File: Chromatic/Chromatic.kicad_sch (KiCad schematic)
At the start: 154 parts

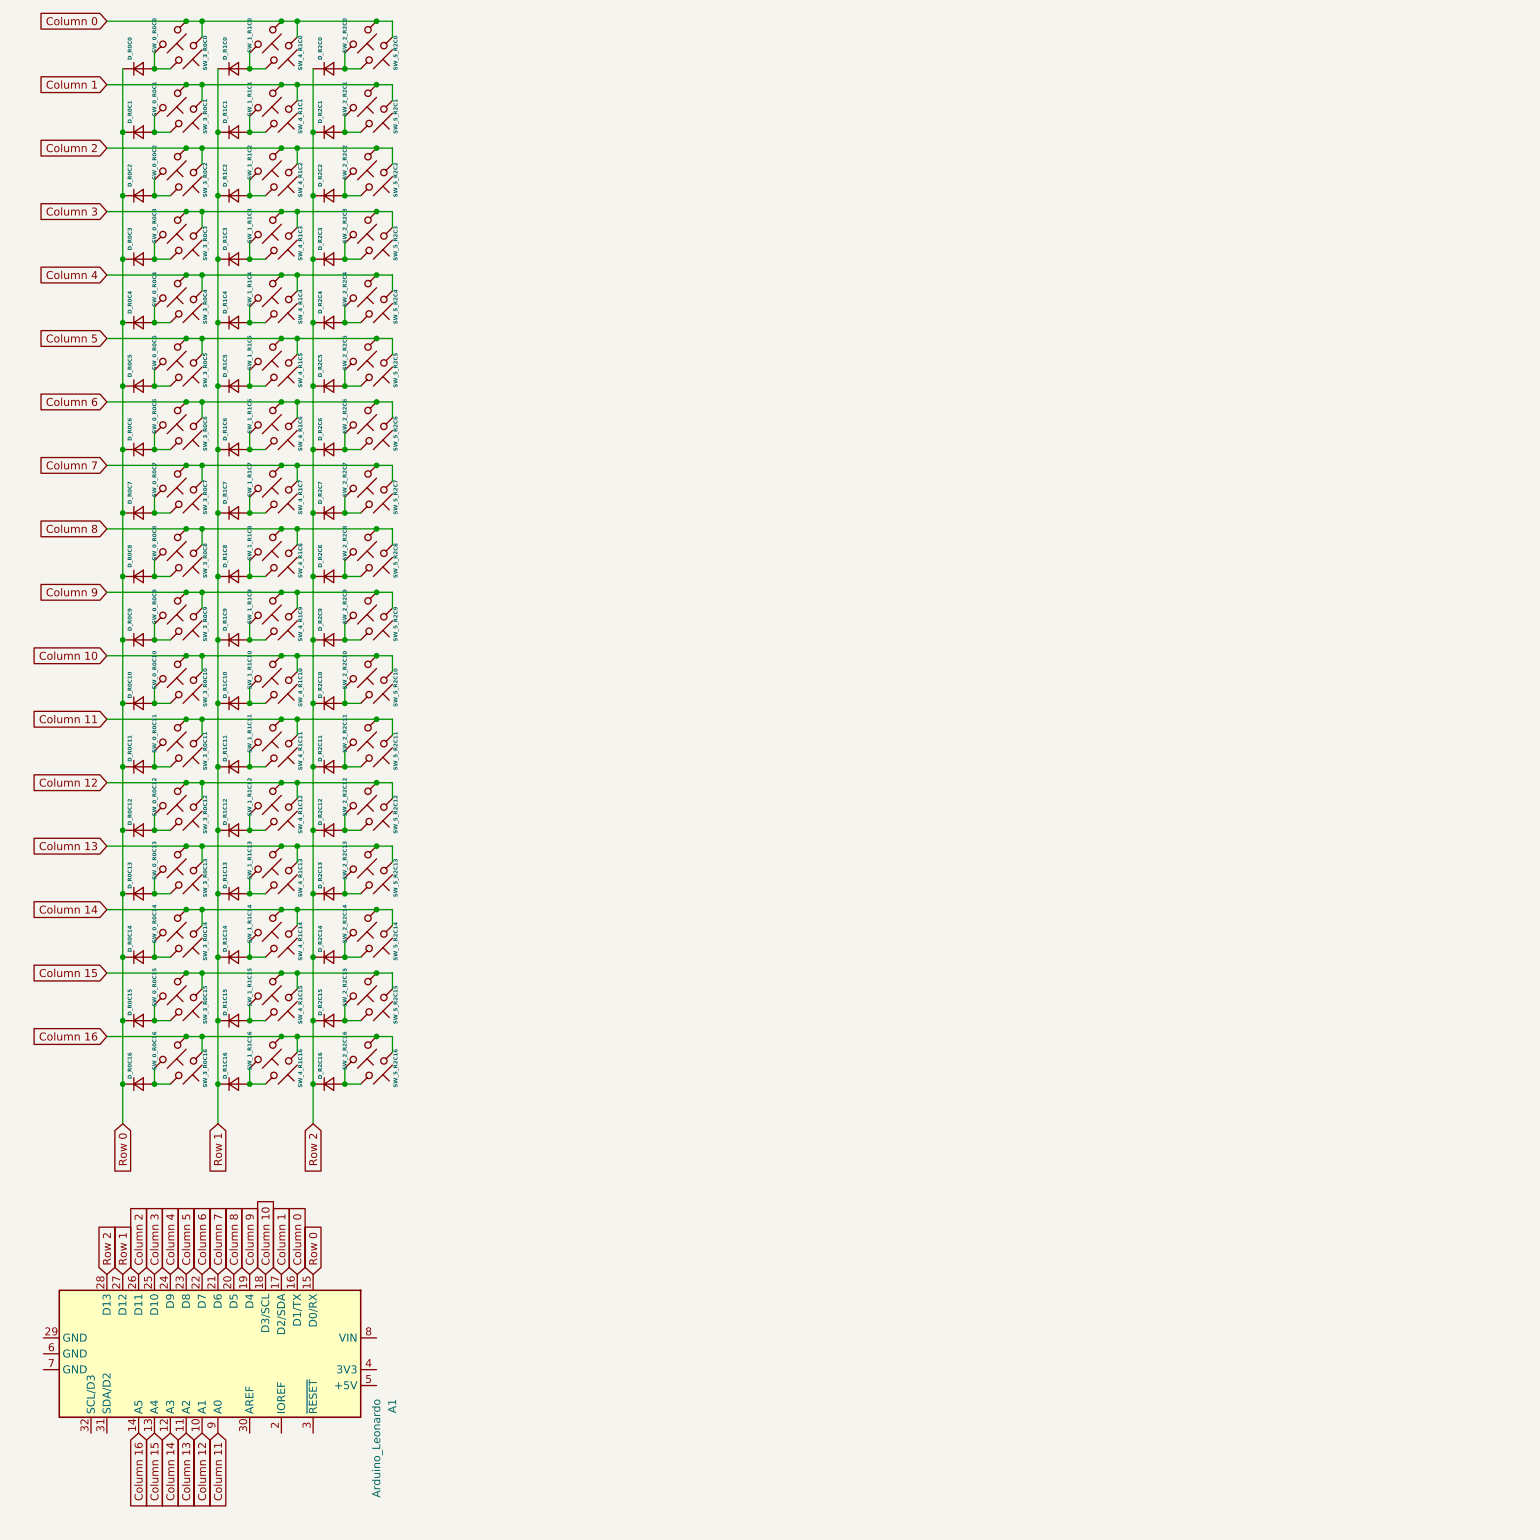
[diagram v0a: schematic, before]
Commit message: octave adjust
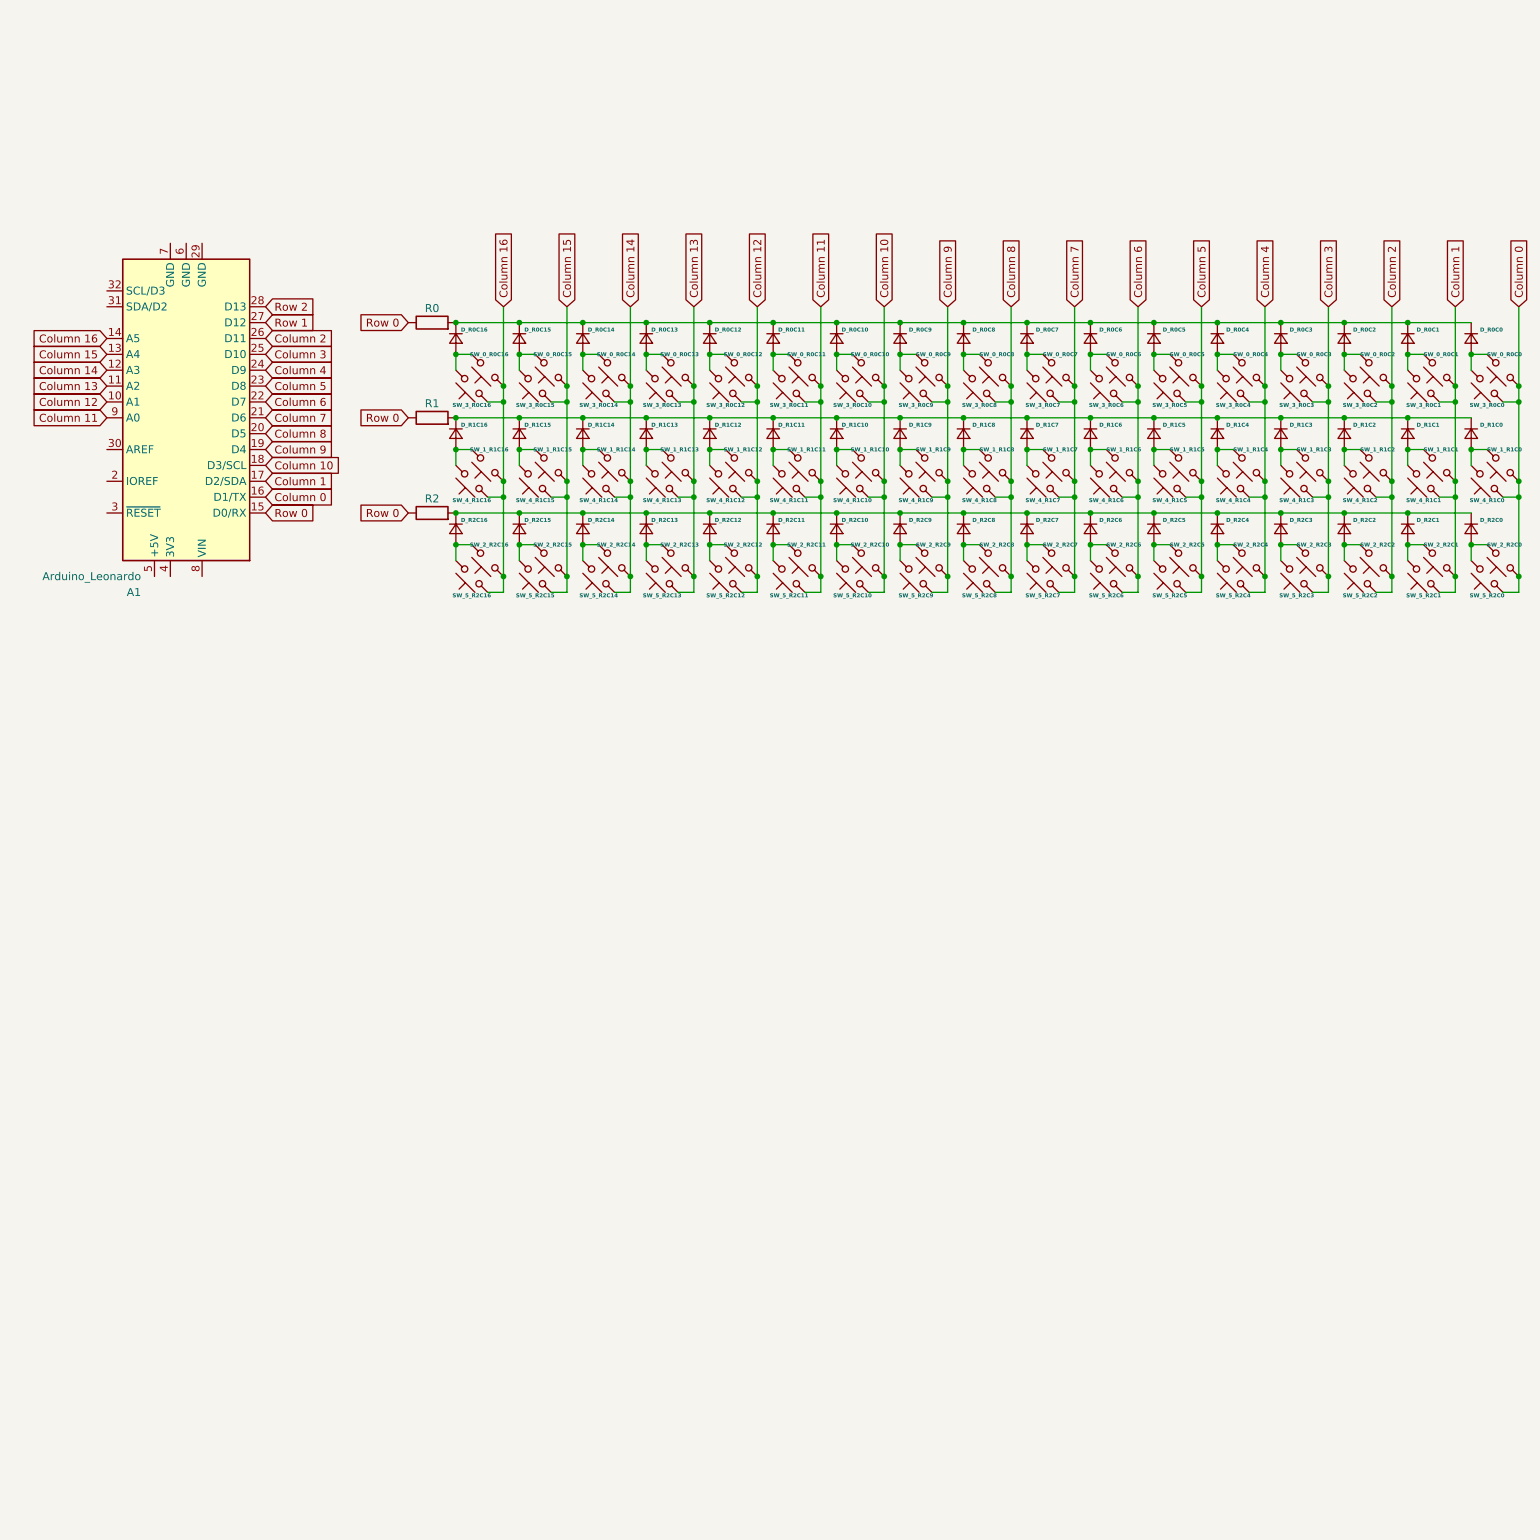
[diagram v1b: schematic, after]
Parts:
- added R0, R1, R2: Resistor, Resistor_THT:R_Axial_DIN0204_L3.6mm_D1.6mm_P5.08mm_Horizontal, symbol ScottoKeebs:Placeholder_Resistor
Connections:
- net Row 0: now also R0.1, R1.1, R2.1; no longer D_R0C0.1 (K), D_R0C1.1 (K), D_R0C10.1 (K), D_R0C11.1 (K), D_R0C12.1 (K), D_R0C13.1 (K), D_R0C14.1 (K), D_R0C15.1 (K), D_R0C16.1 (K), D_R0C2.1 (K), D_R0C3.1 (K), D_R0C4.1 (K), D_R0C5.1 (K), D_R0C6.1 (K), D_R0C7.1 (K), D_R0C8.1 (K), D_R0C9.1 (K)
- net Row 1: no longer D_R1C0.1 (K), D_R1C1.1 (K), D_R1C10.1 (K), D_R1C11.1 (K), D_R1C12.1 (K), D_R1C13.1 (K), D_R1C14.1 (K), D_R1C15.1 (K), D_R1C16.1 (K), D_R1C2.1 (K), D_R1C3.1 (K), D_R1C4.1 (K), D_R1C5.1 (K), D_R1C6.1 (K), D_R1C7.1 (K), D_R1C8.1 (K), D_R1C9.1 (K)
- net Row 2: no longer D_R2C0.1 (K), D_R2C1.1 (K), D_R2C10.1 (K), D_R2C11.1 (K), D_R2C12.1 (K), D_R2C13.1 (K), D_R2C14.1 (K), D_R2C15.1 (K), D_R2C16.1 (K), D_R2C2.1 (K), D_R2C3.1 (K), D_R2C4.1 (K), D_R2C5.1 (K), D_R2C6.1 (K), D_R2C7.1 (K), D_R2C8.1 (K), D_R2C9.1 (K)
- new net: D_R2C0.1 (K), D_R2C1.1 (K), D_R2C10.1 (K), D_R2C11.1 (K), D_R2C12.1 (K), D_R2C13.1 (K), D_R2C14.1 (K), D_R2C15.1 (K), D_R2C16.1 (K), D_R2C2.1 (K), D_R2C3.1 (K), D_R2C4.1 (K), D_R2C5.1 (K), D_R2C6.1 (K), D_R2C7.1 (K), D_R2C8.1 (K), D_R2C9.1 (K), R2.2
- new net: D_R0C0.1 (K), D_R0C1.1 (K), D_R0C10.1 (K), D_R0C11.1 (K), D_R0C12.1 (K), D_R0C13.1 (K), D_R0C14.1 (K), D_R0C15.1 (K), D_R0C16.1 (K), D_R0C2.1 (K), D_R0C3.1 (K), D_R0C4.1 (K), D_R0C5.1 (K), D_R0C6.1 (K), D_R0C7.1 (K), D_R0C8.1 (K), D_R0C9.1 (K), R0.2
- new net: D_R1C0.1 (K), D_R1C1.1 (K), D_R1C10.1 (K), D_R1C11.1 (K), D_R1C12.1 (K), D_R1C13.1 (K), D_R1C14.1 (K), D_R1C15.1 (K), D_R1C16.1 (K), D_R1C2.1 (K), D_R1C3.1 (K), D_R1C4.1 (K), D_R1C5.1 (K), D_R1C6.1 (K), D_R1C7.1 (K), D_R1C8.1 (K), D_R1C9.1 (K), R1.2
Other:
- moved on the sheet: A1, D_R0C0, D_R0C1, D_R0C10, D_R0C11, D_R0C12, D_R0C13, D_R0C14, D_R0C15, D_R0C16, D_R0C2, D_R0C3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
